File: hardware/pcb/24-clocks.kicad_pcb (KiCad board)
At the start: 2 copper layers, 165.1 x 94 mm, 90 parts, among them J201 ST-LINK, J202 Debug UART, J401 Conn_01x04, J402 Conn_01x04, J601 Conn_02x03_Odd_Even, U201 STM32F103C8Tx, U301 VID28-05, U302 VID66-08, U303 AH3572, U304 AH3572, U401 MAX3485, U501 AMS1117-5.0, U502 AMS1117-3.3, U601 ESP32-WROOM-32D, U701 24LC512, U702 DS1307+, Y201 8MHz, Y701 32.768kHz

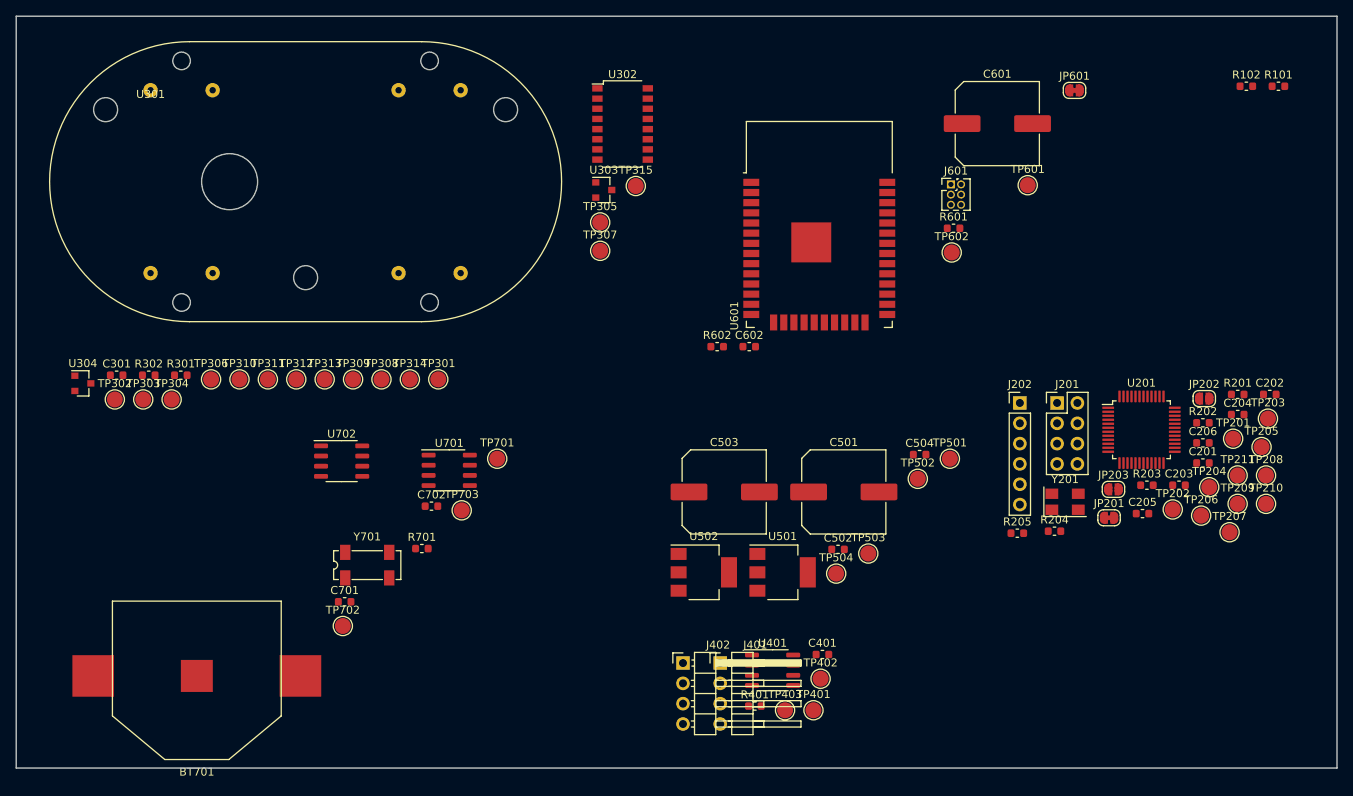
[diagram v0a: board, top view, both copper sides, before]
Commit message: Finished PCB (#3)
* Created PCB outline and first placement

* Changed connectors

* Minor

* Included all 3D files

* Mixed changes

* Changed supply to 7V

* Archived PCB project

* Update 24-clocks-rescue.lib

* First placement

* Routed supplies

* Update 24-clocks.kicad_pcb

* Added routing

* Routed more nets

* Finished routing

* Archived project

* Replace hash and date

* minor

* Update pcb.yml

* Update pcb.yml

* Update pcb.yml

* Update pcb.yml

* Auto update commit date and hash

* Update output

* changed outputs

* Added layer to output

* Update hash and date also in sch

* Added caps to hall sensors

* Cleanup files
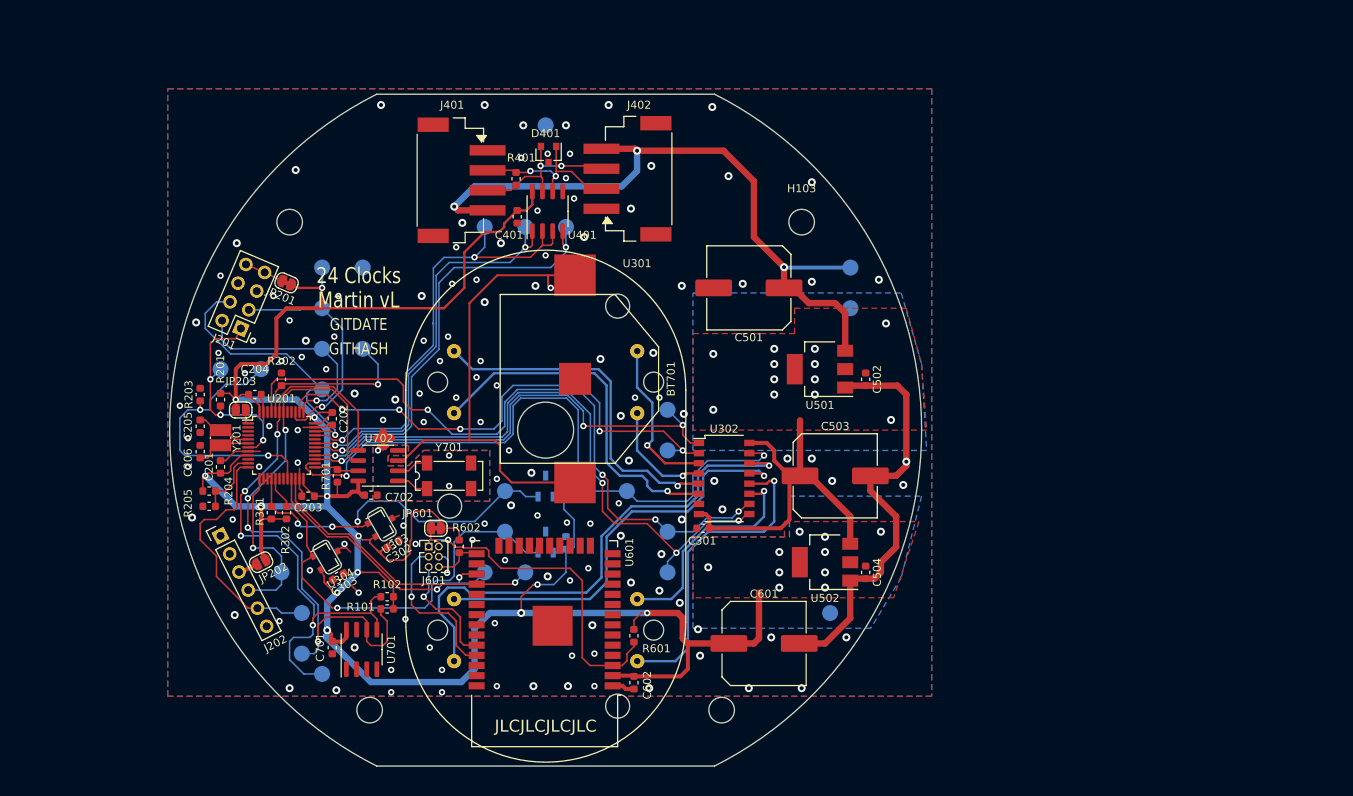
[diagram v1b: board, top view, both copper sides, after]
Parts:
- removed TP211: HW-Version, TestPoint:TestPoint_Pad_D2.0mm
- removed TP301: MA1, TestPoint:TestPoint_Pad_D2.0mm
- removed TP302: MA2, TestPoint:TestPoint_Pad_D2.0mm
- removed TP304: MA3, TestPoint:TestPoint_Pad_D2.0mm
- removed TP307: MA4, TestPoint:TestPoint_Pad_D2.0mm
- removed TP310: MB1, TestPoint:TestPoint_Pad_D2.0mm
- removed TP311: MB2, TestPoint:TestPoint_Pad_D2.0mm
- removed TP312: MB3, TestPoint:TestPoint_Pad_D2.0mm
- removed TP313: MB4, TestPoint:TestPoint_Pad_D2.0mm
- added C302: 100nF, Capacitor_SMD:C_0603_1608Metric, F.Cu at (130.9, 114.2)
- added C303: 100nF, Capacitor_SMD:C_0603_1608Metric, F.Cu at (124.1, 118.3)
- added C304: 100nF, Capacitor_SMD:C_0603_1608Metric, B.Cu at (152.3, 107.0)
- added C305: 100nF, Capacitor_SMD:C_0603_1608Metric, B.Cu at (152.5, 114.1)
- added D401: PESD1CAN, Package_TO_SOT_SMD:SOT-23, F.Cu at (150.4, 65.5)
- added H101: MountingHole, MountingHole:MountingHole_3.2mm_M3, F.Cu at (118.0, 74.0)
- added H102: MountingHole, MountingHole:MountingHole_3.2mm_M3, F.Cu at (172.0, 135.0)
- added H103: MountingHole, MountingHole:MountingHole_3.2mm_M3, F.Cu at (182.0, 74.0)
- added H104: MountingHole, MountingHole:MountingHole_3.2mm_M3, F.Cu at (128.0, 135.0)
- added NT701: Net-Tie_2, NetTie:NetTie-2_SMD_Pad0.5mm, F.Cu at (129.7, 101.5)
- added U305: AH3572, Package_TO_SOT_SMD:TSOT-23, B.Cu at (150.0, 107.0)
- added U306: AH3572, Package_TO_SOT_SMD:TSOT-23, B.Cu at (150.0, 114.0)
- J401, J402: value Conn_01x04 -> S4B_XH_SM4_TB; footprint Connector_PinHeader_2.54mm:PinHeader_1x04_P2.54mm_Horizontal -> mvl-footprints:JST_S4B_XH_SM4_TB
- TP201, TP202, TP203, TP204, TP205, TP206, TP207, TP208, TP209, TP210, TP303, TP305, TP306, TP308, TP309, TP314, TP315, TP401, TP402, TP403, TP501, TP502, TP503, TP504, TP601, TP602, TP701, TP702, TP703: moved to B.Cu
- U301: footprint mvl-footprints:vid_28_05 -> mvl-footprints:BK30D-R5
- U303, U304: footprint Package_TO_SOT_SMD:SOT-23 -> mvl-footprints:SOT-23-UD
- U401, U701, U702: footprint Package_SO:SO-8_3.9x4.9mm_P1.27mm -> Package_SO:SOIC-8_3.9x4.9mm_P1.27mm
- Y201: value 8MHz -> NX3225GD 8MHz; footprint Crystal:Crystal_SMD_5032-4Pin_5.0x3.2mm -> mvl-footprints:Crystal_SMD_3225-2Pin_3.2x2.5mm
- Y701: footprint Crystal:Crystal_SMD_SeikoEpson_MC306-4Pin_8.0x3.2mm -> mvl-footprints:Crystal_SMD_SeikoEpson_MC306-4Pin_8.0x3.2mm
- moved R101 129.2 mm to (130.2, 122.4), turned to 180 degrees
- moved R201 127.2 mm to (109.4, 96.2), turned to 270 degrees
- moved TP208 126.3 mm to (114.4, 92.4)
- moved C206 125.3 mm to (106.8, 102.7), turned to 90 degrees
- moved R102 124.9 mm to (130.2, 120.8), turned to 180 degrees
- moved C204 122.9 mm to (113.7, 95.6)
- moved C201 122.8 mm to (109.4, 104.6), turned to 90 degrees
- moved TP210 121.3 mm to (119.5, 122.9)
- moved TP202 120.3 mm to (109.4, 92.4)
- moved TP209 119.8 mm to (117.0, 117.8)
- moved JP202 119.7 mm to (114.4, 116.5), turned to 207 degrees
- moved TP205 119.6 mm to (122.1, 79.7)
- moved R203 118.9 mm to (106.8, 95.6), turned to 90 degrees
- moved TP203 118.6 mm to (122.1, 89.8)
- moved C205 118.3 mm to (106.8, 99.5), turned to 270 degrees
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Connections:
- net +9V renamed +7.5V
- net Net-(BT701-Pad1) renamed /RTC and Memory/Vbat
- C702 pad 2: GND -> /RTC and Memory/GND-CLK
- R701 pad 2: /RTC and Memory/RCLK -> /RTC and Memory/RTC-CLK
- U201 pad 25: (no net) -> /RTC and Memory/RTC-CLK
- U702 pad 4: GND -> /RTC and Memory/GND-CLK
- U702 pad 7: /RTC and Memory/RCLK -> /RTC and Memory/RTC-CLK
- Y201 pad 2: GND -> Net-(C206-Pad1)
- Y701 pad 2: GND -> /RTC and Memory/GND-CLK
- Y701 pad 3: GND -> /RTC and Memory/GND-CLK
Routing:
- net +3V3: track 0.00 -> 323.4 mm, vias 0 -> 23
- net +7.5V: track 0.00 -> 89.2 mm, vias 0 -> 3
- net /Mechanics/M-A-Step: track 0.00 -> 86.9 mm, vias 0 -> 4
- net /Mechanics/M-Rst: track 0.00 -> 82.5 mm, vias 0 -> 2
- net GND: track 0.00 -> 82.1 mm, vias 0 -> 134
- net /Mechanics/M-A-CW: track 0.00 -> 79.1 mm, vias 0 -> 4
- net /I2C-SDA: track 0.00 -> 78.8 mm, vias 0 -> 4
- net /I2C-SCL: track 0.00 -> 77.4 mm, vias 0 -> 4
- net /Mechanics/M-B-Step: track 0.00 -> 64.9 mm, vias 0 -> 5
- net /Mechanics/MB3: track 0.00 -> 64.6 mm, vias 0 -> 1
- net /RTC and Memory/Vbat: track 0.00 -> 62.6 mm, vias 0 -> 1
- net /Mechanics/M-B-CW: track 0.00 -> 60.7 mm, vias 0 -> 3
- net /Com Bus/uC-RS485-DE: track 0.00 -> 57.5 mm, vias 0 -> 2
- net /Com Bus/uC-RS485-Tx: track 0.00 -> 55.7 mm, vias 0 -> 2
- net /Mechanics/HAL-B: track 0.00 -> 55.2 mm, vias 0 -> 1
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- added copper zone on B.Cu, net +3V3
- added copper zone on F.Cu, net +3V3
- added copper zone on B.Cu, net +5V
- added copper zone on F.Cu, net +5V
- added copper zone on F.Cu, net /RTC and Memory/GND-CLK
- added copper zone on B.Cu, net /RTC and Memory/RTC-CLK
- added copper zone on B.Cu, net GND
- added copper zone on F.Cu, net GND
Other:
- board size 165.1 x 94 mm -> 94 x 84 mm
- net class Default: clearance 0.2 -> 0.15; trace_width 0.25 -> 0.2
- net class Motor added: clearance 0.2, trace_width 0.3, via_dia 0.8, via_drill 0.4
- net class Power added: clearance 0.2, trace_width 0.5, via_dia 1, via_drill 0.5
- net class RS485 added: clearance 0.2, trace_width 0.3, via_dia 0.8, via_drill 0.4
- rule pad_to_mask_clearance: 0.051 -> 0
- rule trace_clearance: 0.2 -> 0.15
- board text added: "24 Clocks"
- board text added: "GITDATE"
- board text added: "GITHASH"
- board text added: "JLCJLCJLCJLC"
- board text added: "Martin vL"

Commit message: Steppers running + pass through master
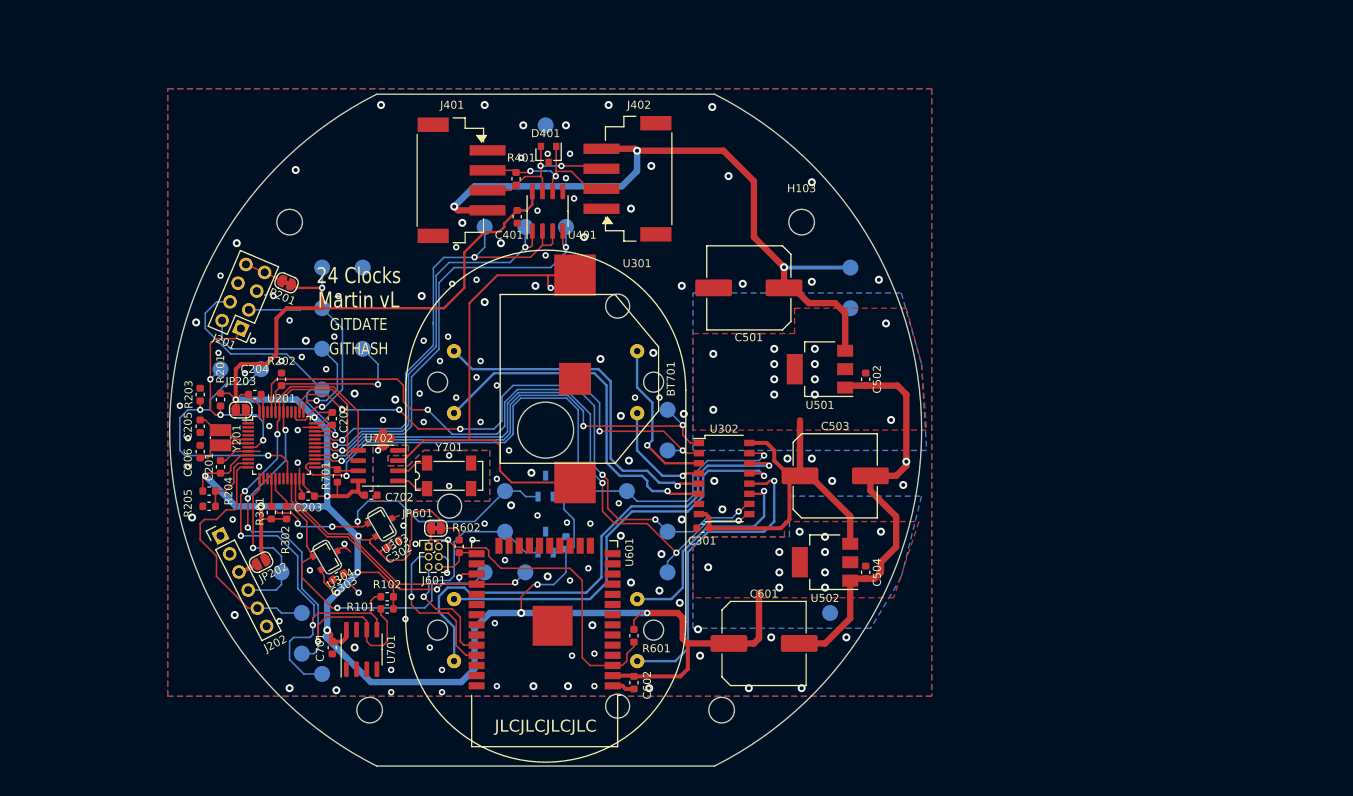
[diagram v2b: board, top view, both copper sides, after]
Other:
- net class Default removed
- net class Motor removed
- net class Power removed
- net class RS485 removed
